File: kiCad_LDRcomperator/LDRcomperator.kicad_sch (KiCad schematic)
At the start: 9 parts, among them J1 Screw_Terminal_01x02

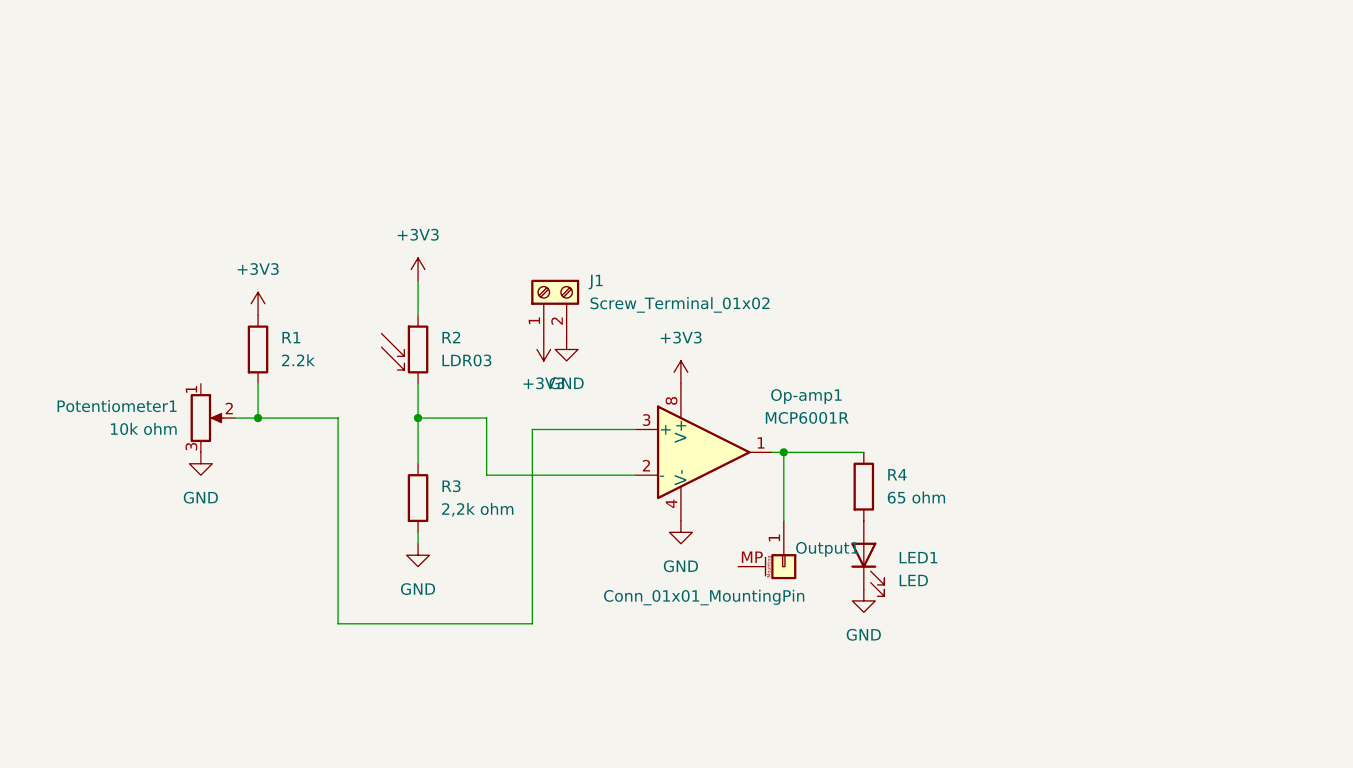
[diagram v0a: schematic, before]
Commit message: updated the LDRComperator kicad drawing
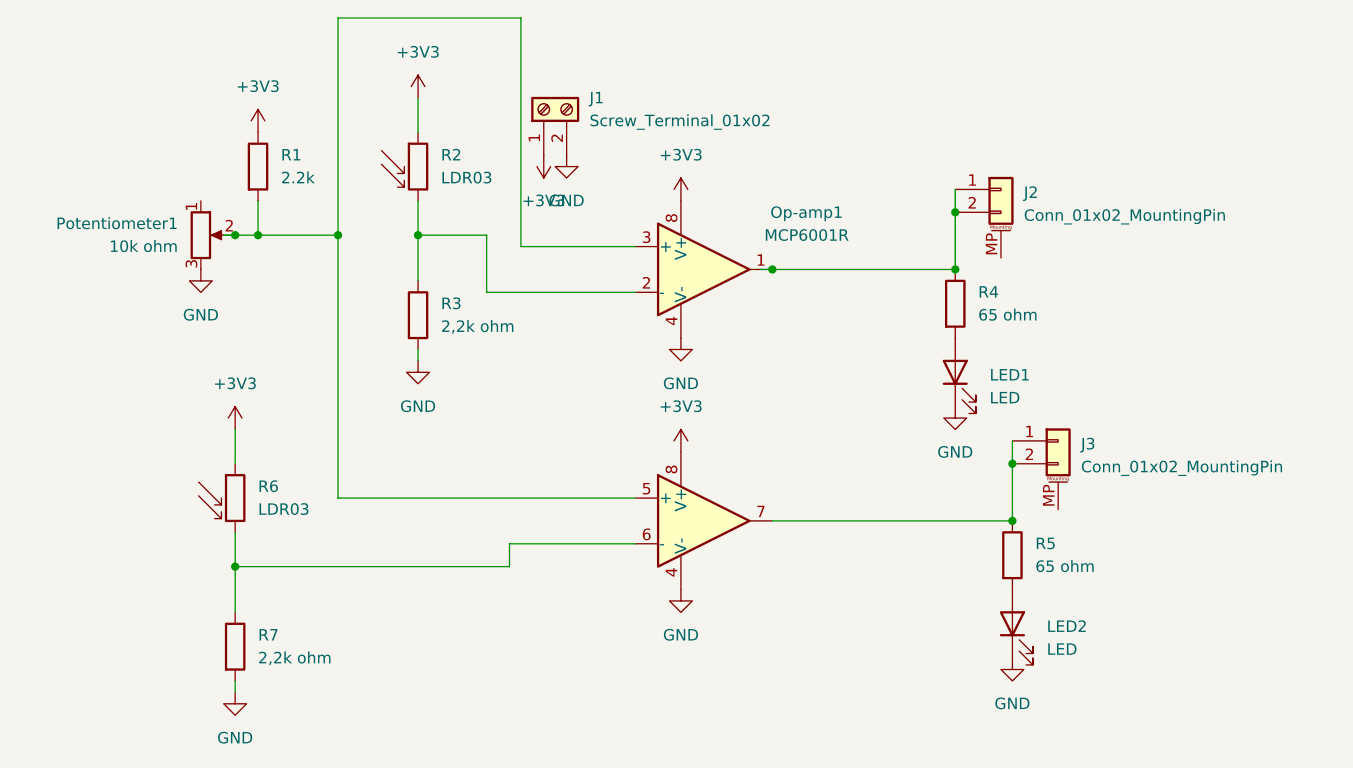
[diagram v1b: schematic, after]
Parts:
- removed Output1: Conn_01x01_MountingPin, Connector_PinSocket_2.54mm:PinSocket_1x01_P2.54mm_Vertical, symbol Connector_Generic_MountingPin:Conn_01x01_MountingPin
- added J2, J3: Conn_01x02_MountingPin, Connector_PinSocket_2.54mm:PinSocket_1x02_P2.54mm_Vertical, symbol Connector_Generic_MountingPin:Conn_01x02_MountingPin
- added LED2: LED, LED_THT:LED_D1.8mm_W3.3mm_H2.4mm, symbol Device:LED
- added R5: 65 ohm, Resistor_THT:R_Axial_DIN0204_L3.6mm_D1.6mm_P7.62mm_Horizontal, symbol Device:R
- added R6: LDR03, TerminalBlock_Phoenix:TerminalBlock_Phoenix_MKDS-1,5-2_1x02_P5.00mm_Horizontal, symbol Sensor_Optical:LDR03
- added R7: 2,2k ohm, Resistor_THT:R_Axial_DIN0204_L3.6mm_D1.6mm_P7.62mm_Horizontal, symbol Device:R
- J1, R2: footprint Connector_PinSocket_2.54mm:PinSocket_1x02_P2.54mm_Vertical -> TerminalBlock_Phoenix:TerminalBlock_Phoenix_MKDS-1,5-2_1x02_P5.00mm_Horizontal
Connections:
- net +3V3: now also R6.1
- net GND: now also LED2.1 (K), R7.2
- net at Op-amp1.1, R4.1: now also J2.1 (Pin_1), J2.2 (Pin_2)
- net at Op-amp1.3 (+), Potentiometer1.2, R1.2: now also Op-amp1.5 (+)
- new net: LED2.2 (A), R5.2
- new net: Op-amp1.6 (-), R6.2, R7.1
- new net: J3.1 (Pin_1), J3.2 (Pin_2), Op-amp1.7, R5.1
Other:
- moved on the sheet: J1, LED1, Potentiometer1, R1, R2, R3, R4
